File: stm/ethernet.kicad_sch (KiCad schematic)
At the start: 4 parts, among them U3 LAN8742A, Y1 25M

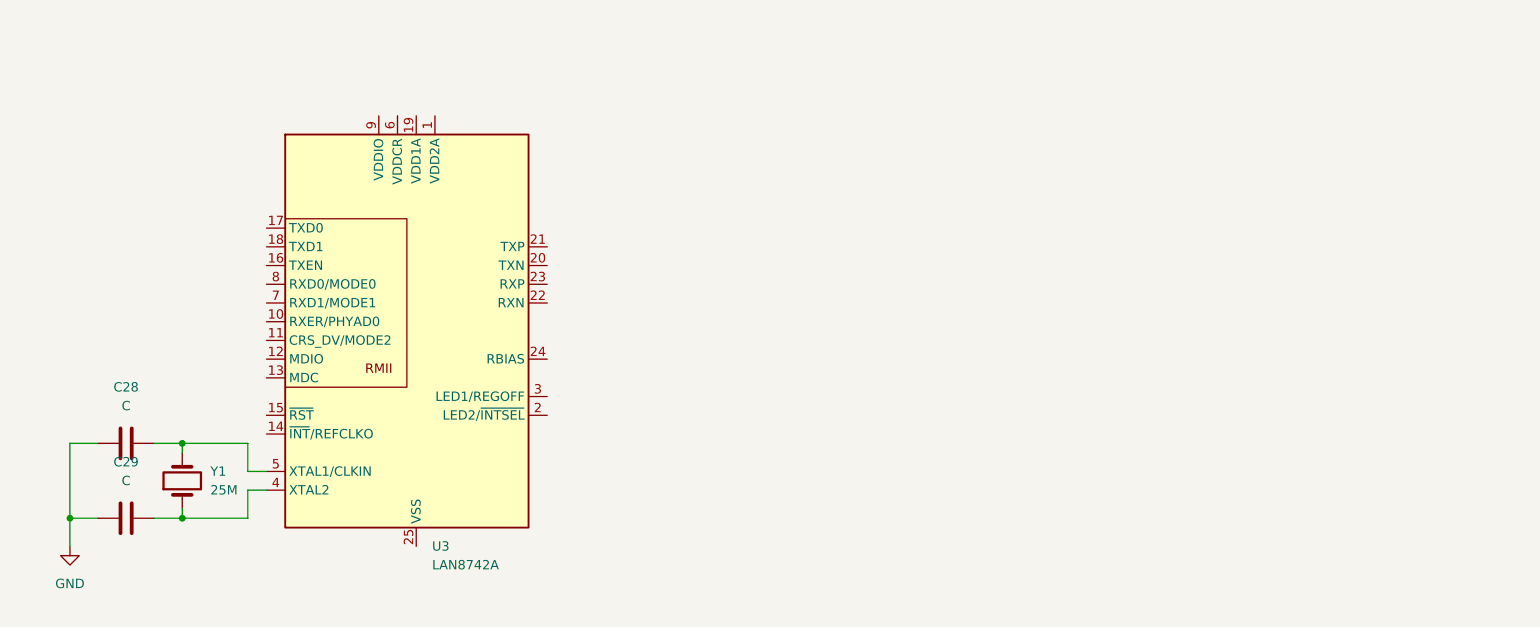
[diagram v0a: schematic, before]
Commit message: ethernet phy
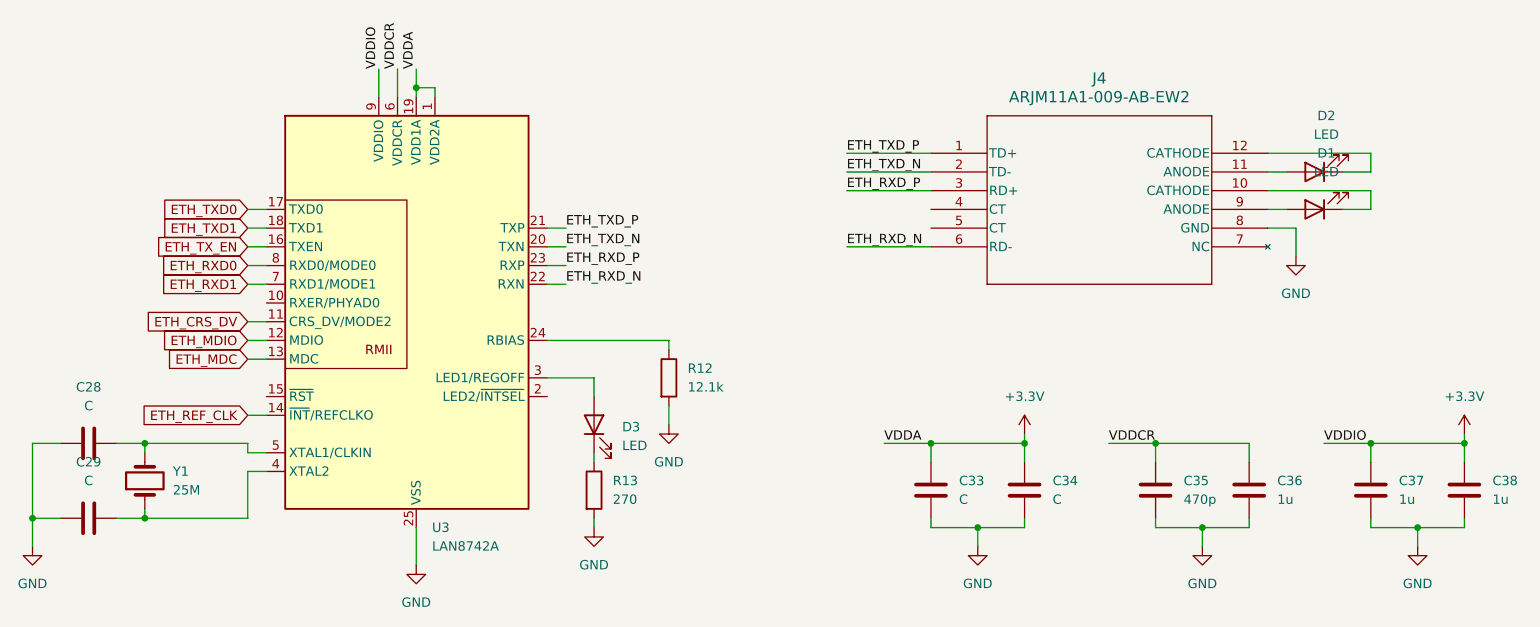
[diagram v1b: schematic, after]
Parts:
- added C33, C34: C, symbol Device:C
- added C35: 470p, symbol Device:C
- added C36, C37, C38: 1u, symbol Device:C
- added D1, D2, D3: LED, symbol Device:LED
- added J4: ARJM11A1-009-AB-EW2, ARJM11A1-009-AB-EW2_ABR, symbol ARJM11A1-009-AB-EW2:ARJM11A1-009-AB-EW2
- added R12: 12.1k, symbol Device:R
- added R13: 270, symbol Device:R
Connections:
- net GND: now also U3.25 (VSS), C33.2, C34.2, C35.2, C36.2, C37.2, C38.2, J4.8 (GND), R12.2, R13.2
- net +3.3V: now reaches U3.1 (VDD2A)
- net +3.3V: now also U3.19 (VDD1A), U3.9 (VDDIO), C33.1, C34.1, C37.1, C38.1
- net ETH_CRS_DV: now reaches U3.11 (CRS_DV/MODE2)
- net ETH_MDIO: now reaches U3.12 (MDIO)
- net ETH_MDC: now reaches U3.13 (MDC)
- net ETH_REF_CLK: now reaches U3.14 (~{INT}/REFCLKO)
- net ETH_TX_EN: now reaches U3.16 (TXEN)
- net ETH_TXD0: now reaches U3.17 (TXD0)
- net ETH_TXD1: now reaches U3.18 (TXD1)
- net ETH_TXD_N: now reaches U3.20 (TXN)
- net ETH_TXD_N: now also J4.2 (TD-)
- net ETH_TXD_P: now reaches U3.21 (TXP)
- net ETH_TXD_P: now also J4.1 (TD+)
- net ETH_RXD_N: now reaches U3.22 (RXN)
- net ETH_RXD_N: now also J4.6 (RD-)
- net ETH_RXD_P: now reaches U3.23 (RXP)
- net ETH_RXD_P: now also J4.3 (RD+)
- net at U3.24 (RBIAS): now also R12.1
- net at U3.3 (LED1/REGOFF): now also D3.2 (A)
- net VDDCR: now reaches U3.6 (VDDCR)
- net VDDCR: now also C35.1, C36.1
- net ETH_RXD1: now reaches U3.7 (RXD1/MODE1)
- net ETH_RXD0: now reaches U3.8 (RXD0/MODE0)
- new net: D3.1 (K), R13.1
- new net: D2.1 (K), J4.12 (CATHODE)
- new net: D2.2 (A), J4.11 (ANODE)
- new net: D1.1 (K), J4.10 (CATHODE)
- new net: D1.2 (A), J4.9 (ANODE)
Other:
- moved on the sheet: C28, C29, U3, Y1
